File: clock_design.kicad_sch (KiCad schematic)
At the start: 30 parts, among them J1 Power_inlet_vertical, U1 ATmega328-PU, U2 L7805, U3 DS1307_DIP-8, Y1 Crystal_16MHz, Y2 Crystal_32768Hz

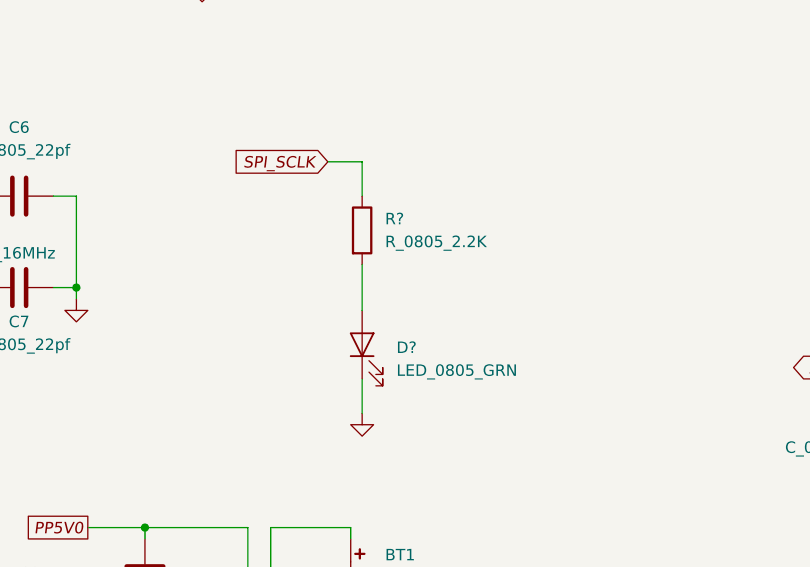
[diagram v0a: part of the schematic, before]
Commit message: Routing in progress...
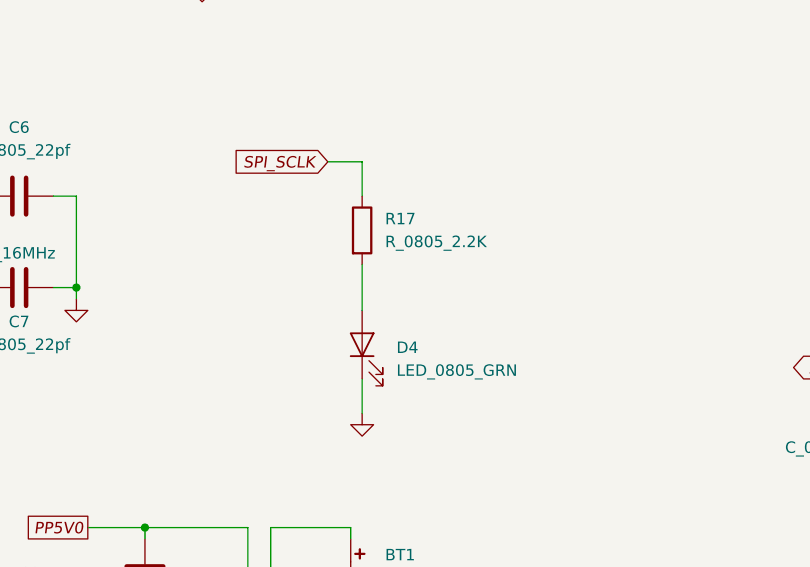
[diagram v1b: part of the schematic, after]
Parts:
- gave numbers to parts that had none: 2
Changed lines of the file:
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@@
   (symbol (lib_id "HPS:GND") (at 139.7 139.7 0) (unit 1)
     (in_bom yes) (on_board yes) (fields_autoplaced)
-    (property "Reference" "#PWR?" (id 0) (at 139.7 146.05 0)
+    (property "Reference" "#PWR0124" (id 0) (at 139.7 146.05 0)
       (effects (font (size 1.27 1.27)) hide)
     )
@@
   (symbol (lib_id "HPS:LED_0805_GRN") (at 139.7 132.08 90) (unit 1)
     (in_bom yes) (on_board yes) (fields_autoplaced)
-    (property "Reference" "D?" (id 0) (at 143.51 132.4101 90)
+    (property "Reference" "D4" (id 0) (at 143.51 132.4101 90)
       (effects (font (size 1.27 1.27)) (justify right))
     )
@@
   (symbol (lib_id "HPS:R_0805_2.2K") (at 139.7 119.38 0) (unit 1)
     (in_bom yes) (on_board yes) (fields_autoplaced)
-    (property "Reference" "R?" (id 0) (at 142.24 118.1099 0)
+    (property "Reference" "R17" (id 0) (at 142.24 118.1099 0)
       (effects (font (size 1.27 1.27)) (justify left))
     )
@@
       (reference "#PWR0123") (unit 1) (value "GND") (footprint "")
     )
+    (path "/1db71ecb-f082-4fe1-8e62-514bcfaa0e2d"
+      (reference "#PWR0124") (unit 1) (value "GND") (footprint "")
+    )
     (path "/398dcb48-e636-4c28-8701-b4906ea4df14/dba4083a-e1a5-423f-9fef-86e5703e621a"
       (reference "#PWR0125") (unit 1) (value "GND") (footprint "")
@@
       (reference "#PWR0136") (unit 1) (value "GND") (footprint "")
     )
-    (path "/1db71ecb-f082-4fe1-8e62-514bcfaa0e2d"
-      (reference "#PWR?") (unit 1) (value "GND") (footprint "")
-    )
     (path "/12399143-5f74-45ac-8086-3f780cf2c591"
       (reference "BT1") (unit 1) (value "Battery_Cell") (footprint "footprints:BatteryHolder_Keystone_106_1x20mm")
@@
     )
     (path "/6e5c2306-97c3-4235-b971-b2ebb60a6cd6"
-      (reference "D?") (unit 1) (value "LED_0805_GRN") (footprint "footprints:LED_0805_2012Metric")
+      (reference "D4") (unit 1) (value "LED_0805_GRN") (footprint "footprints:LED_0805_2012Metric")
     )
     (path "/e73d99b1-0f17-4396-814b-a78c0ffe84da/8d63d620-db80-4923-8b2e-4dba06f0aba5"
@@
       (reference "R16") (unit 1) (value "R_0805_22K") (footprint "footprints:R_0805_2012Metric")
     )
+    (path "/b5ae2498-fe7c-40d9-922a-566679c1819f"
+      (reference "R17") (unit 1) (value "R_0805_2.2K") (footprint "footprints:R_0805_2012Metric")
+    )
     (path "/61bf49de-7bf3-4092-92f7-a9f338e64263/13c76214-6134-446b-8d07-3a965a1923e5"
       (reference "R18") (unit 1) (value "R_0805_22K") (footprint "footprints:R_0805_2012Metric")
@@
       (reference "R23") (unit 1) (value "R_0805_47") (footprint "footprints:R_0805_2012Metric")
     )
-    (path "/b5ae2498-fe7c-40d9-922a-566679c1819f"
-      (reference "R?") (unit 1) (value "R_0805_2.2K") (footprint "footprints:R_0805_2012Metric")
-    )
     (path "/1ded9e65-d766-4467-8652-a295879c8ab2/aa99d72d-ef0a-4c0c-95ca-bb3964a1ede7"
